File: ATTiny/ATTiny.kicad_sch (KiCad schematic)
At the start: 6 parts

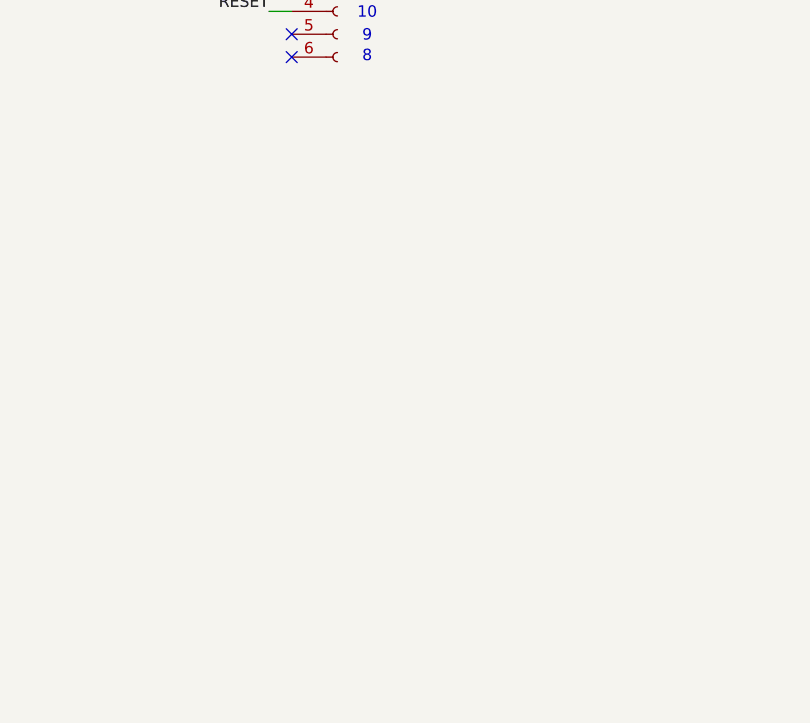
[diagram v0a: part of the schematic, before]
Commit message: header pins complete
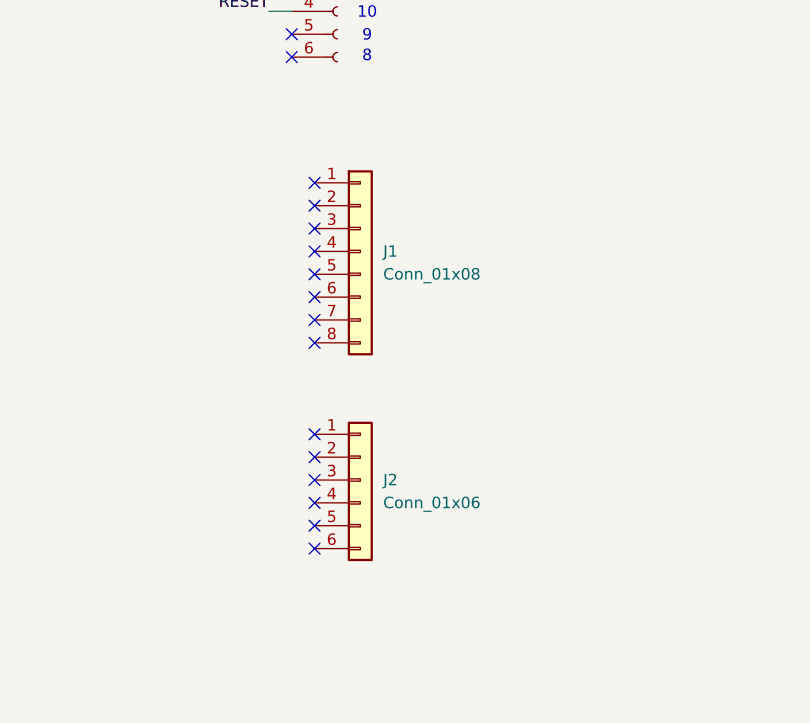
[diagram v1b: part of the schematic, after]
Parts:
- added J1: Conn_01x08, symbol Connector_Generic:Conn_01x08
- added J2: Conn_01x06, symbol Connector_Generic:Conn_01x06
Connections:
- no-connect marks 6 -> 20
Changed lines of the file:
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@@
+	)
+	(no_connect
+		(at 102.87 77.47)
+	)
+	(no_connect
+		(at 102.87 74.93)
+	)
+	(no_connect
+		(at 102.87 92.71)
+	)
+	(no_connect
+		(at 102.87 87.63)
+	)
+	(no_connect
+		(at 102.87 67.31)
+	)
+	(no_connect
+		(at 102.87 95.25)
 	)
 	(no_connect
@@
 	)
 	(no_connect
+		(at 102.87 69.85)
+	)
+	(no_connect
+		(at 102.87 59.69)
+	)
+	(no_connect
+		(at 102.87 97.79)
+	)
+	(no_connect
+		(at 102.87 72.39)
+	)
+	(no_connect
 		(at 33.02 45.72)
 	)
 	(no_connect
+		(at 102.87 64.77)
+	)
+	(no_connect
 		(at 34.29 90.17)
 	)
 	(no_connect
 		(at 34.29 92.71)
+	)
+	(no_connect
+		(at 102.87 62.23)
+	)
+	(no_connect
+		(at 102.87 90.17)
+	)
+	(no_connect
+		(at 102.87 100.33)
 	)
 	(wire
@@
 					(unit 1)
 				)
+			)
+		)
+	)
+	(symbol
+		(lib_id "Connector_Generic:Conn_01x06")
+		(at 107.95 92.71 0)
+		(unit 1)
+		(body_style 1)
+		(exclude_from_sim no)
+		(in_bom yes)
+		(on_board yes)
+		(in_pos_files yes)
+		(dnp no)
+		(fields_autoplaced yes)
+		(property "Reference" "J2"
+			(at 110.49 92.7099 0)
+			(show_name no)
+			(do_not_autoplace no)
+			(effects
+				(font
+					(size 1.27 1.27)
+				)
+				(justify left)
+			)
+		)
+		(property "Value" "Conn_01x06"
+			(at 110.49 95.2499 0)
+			(show_name no)
+			(do_not_autoplace no)
+			(effects
+				(font
+					(size 1.27 1.27)
+				)
+				(justify left)
+			)
+		)
+		(property "Footprint" ""
+			(at 107.95 92.71 0)
+			(hide yes)
+			(show_name no)
+			(do_not_autoplace no)
+			(effects
+				(font
+					(size 1.27 1.27)
+				)
+			)
+		)
+		(property "Datasheet" ""
+			(at 107.95 92.71 0)
+			(hide yes)
+			(show_name no)
+			(do_not_autoplace no)
+			(effects
+				(font
+					(size 1.27 1.27)
+				)
+			)
+		)
+		(property "Description" "Generic connector, single row, 01x06, script generated (kicad-library-utils/schlib/autogen/connector/)"
+			(at 107.95 92.71 0)
+			(hide yes)
+			(show_name no)
+			(do_not_autoplace no)
+			(effects
+				(font
+					(size 1.27 1.27)
+				)
+			)
+		)
+		(pin "3"
+		)
+		(pin "2"
+		)
+		(pin "1"
+		)
+		(pin "4"
+		)
+		(pin "6"
+		)
+		(pin "5"
+		)
+		(instances
+			(project "ATTiny"
+				(path "/46ef1815-a8ed-4d38-a82f-c72395c084aa"
+					(reference "J2")
+					(unit 1)
+				)
+			)
+		)
+	)
+	(symbol
+		(lib_id "Connector_Generic:Conn_01x08")
+		(at 107.95 67.31 0)
+		(unit 1)
+		(body_style 1)
+		(exclude_from_sim no)
+		(in_bom yes)
+		(on_board yes)
+		(in_pos_files yes)
+		(dnp no)
+		(fields_autoplaced yes)
+		(property "Reference" "J1"
+			(at 110.49 67.3099 0)
+			(show_name no)
+			(do_not_autoplace no)
+			(effects
+				(font
+					(size 1.27 1.27)
+				)
+				(justify left)
+			)
+		)
+		(property "Value" "Conn_01x08"
+			(at 110.49 69.8499 0)
+			(show_name no)
+			(do_not_autoplace no)
+			(effects
+				(font
+					(size 1.27 1.27)
+				)
+				(justify left)
+			)
+		)
+		(property "Footprint" ""
+			(at 107.95 67.31 0)
+			(hide yes)
+			(show_name no)
+			(do_not_autoplace no)
+			(effects
+				(font
+					(size 1.27 1.27)
+				)
+			)
+		)
+		(property "Datasheet" ""
+			(at 107.95 67.31 0)
+			(hide yes)
+			(show_name no)
+			(do_not_autoplace no)
+			(effects
+				(font
+					(size 1.27 1.27)
+				)
+			)
+		)
+		(property "Description" "Generic connector, single row, 01x08, script generated (kicad-library-utils/schlib/autogen/connector/)"
+			(at 107.95 67.31 0)
+			(hide yes)
+			(show_name no)
+			(do_not_autoplace no)
+			(effects
+				(font
+					(size 1.27 1.27)
+				)
+			)
+		)
+		(pin "8"
+		)
+		(pin "7"
+		)
+		(pin "5"
+		)
+		(pin "4"
+		)
+		(pin "1"
+		)
+		(pin "3"
+		)
+		(pin "2"
+		)
+		(pin "6"
+		)
+		(instances
+			(project "ATTiny"
+				(path "/46ef1815-a8ed-4d38-a82f-c72395c084aa"
+					(reference "J1")
+					(unit 1)
+				)

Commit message: return
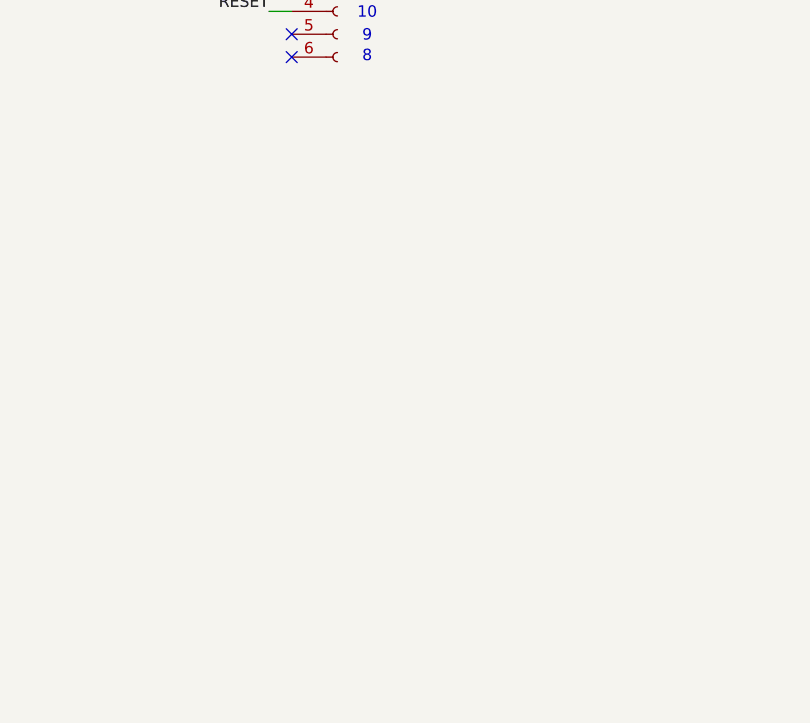
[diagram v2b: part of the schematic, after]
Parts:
- removed J1: Conn_01x08, symbol Connector_Generic:Conn_01x08
- removed J2: Conn_01x06, symbol Connector_Generic:Conn_01x06
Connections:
- no-connect marks 20 -> 6
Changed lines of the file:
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@@
-	)
-	(no_connect
-		(at 102.87 77.47)
-	)
-	(no_connect
-		(at 102.87 74.93)
-	)
-	(no_connect
-		(at 102.87 92.71)
-	)
-	(no_connect
-		(at 102.87 87.63)
-	)
-	(no_connect
-		(at 102.87 67.31)
-	)
-	(no_connect
-		(at 102.87 95.25)
 	)
 	(no_connect
@@
 	)
 	(no_connect
-		(at 102.87 69.85)
-	)
-	(no_connect
-		(at 102.87 59.69)
-	)
-	(no_connect
-		(at 102.87 97.79)
-	)
-	(no_connect
-		(at 102.87 72.39)
-	)
-	(no_connect
 		(at 33.02 45.72)
-	)
-	(no_connect
-		(at 102.87 64.77)
 	)
 	(no_connect
@@
 	(no_connect
 		(at 34.29 92.71)
-	)
-	(no_connect
-		(at 102.87 62.23)
-	)
-	(no_connect
-		(at 102.87 90.17)
-	)
-	(no_connect
-		(at 102.87 100.33)
 	)
 	(wire
@@
 					(unit 1)
 				)
-			)
-		)
-	)
-	(symbol
-		(lib_id "Connector_Generic:Conn_01x06")
-		(at 107.95 92.71 0)
-		(unit 1)
-		(body_style 1)
-		(exclude_from_sim no)
-		(in_bom yes)
-		(on_board yes)
-		(in_pos_files yes)
-		(dnp no)
-		(fields_autoplaced yes)
-		(property "Reference" "J2"
-			(at 110.49 92.7099 0)
-			(show_name no)
-			(do_not_autoplace no)
-			(effects
-				(font
-					(size 1.27 1.27)
-				)
-				(justify left)
-			)
-		)
-		(property "Value" "Conn_01x06"
-			(at 110.49 95.2499 0)
-			(show_name no)
-			(do_not_autoplace no)
-			(effects
-				(font
-					(size 1.27 1.27)
-				)
-				(justify left)
-			)
-		)
-		(property "Footprint" ""
-			(at 107.95 92.71 0)
-			(hide yes)
-			(show_name no)
-			(do_not_autoplace no)
-			(effects
-				(font
-					(size 1.27 1.27)
-				)
-			)
-		)
-		(property "Datasheet" ""
-			(at 107.95 92.71 0)
-			(hide yes)
-			(show_name no)
-			(do_not_autoplace no)
-			(effects
-				(font
-					(size 1.27 1.27)
-				)
-			)
-		)
-		(property "Description" "Generic connector, single row, 01x06, script generated (kicad-library-utils/schlib/autogen/connector/)"
-			(at 107.95 92.71 0)
-			(hide yes)
-			(show_name no)
-			(do_not_autoplace no)
-			(effects
-				(font
-					(size 1.27 1.27)
-				)
-			)
-		)
-		(pin "3"
-		)
-		(pin "2"
-		)
-		(pin "1"
-		)
-		(pin "4"
-		)
-		(pin "6"
-		)
-		(pin "5"
-		)
-		(instances
-			(project "ATTiny"
-				(path "/46ef1815-a8ed-4d38-a82f-c72395c084aa"
-					(reference "J2")
-					(unit 1)
-				)
-			)
-		)
-	)
-	(symbol
-		(lib_id "Connector_Generic:Conn_01x08")
-		(at 107.95 67.31 0)
-		(unit 1)
-		(body_style 1)
-		(exclude_from_sim no)
-		(in_bom yes)
-		(on_board yes)
-		(in_pos_files yes)
-		(dnp no)
-		(fields_autoplaced yes)
-		(property "Reference" "J1"
-			(at 110.49 67.3099 0)
-			(show_name no)
-			(do_not_autoplace no)
-			(effects
-				(font
-					(size 1.27 1.27)
-				)
-				(justify left)
-			)
-		)
-		(property "Value" "Conn_01x08"
-			(at 110.49 69.8499 0)
-			(show_name no)
-			(do_not_autoplace no)
-			(effects
-				(font
-					(size 1.27 1.27)
-				)
-				(justify left)
-			)
-		)
-		(property "Footprint" ""
-			(at 107.95 67.31 0)
-			(hide yes)
-			(show_name no)
-			(do_not_autoplace no)
-			(effects
-				(font
-					(size 1.27 1.27)
-				)
-			)
-		)
-		(property "Datasheet" ""
-			(at 107.95 67.31 0)
-			(hide yes)
-			(show_name no)
-			(do_not_autoplace no)
-			(effects
-				(font
-					(size 1.27 1.27)
-				)
-			)
-		)
-		(property "Description" "Generic connector, single row, 01x08, script generated (kicad-library-utils/schlib/autogen/connector/)"
-			(at 107.95 67.31 0)
-			(hide yes)
-			(show_name no)
-			(do_not_autoplace no)
-			(effects
-				(font
-					(size 1.27 1.27)
-				)
-			)
-		)
-		(pin "8"
-		)
-		(pin "7"
-		)
-		(pin "5"
-		)
-		(pin "4"
-		)
-		(pin "1"
-		)
-		(pin "3"
-		)
-		(pin "2"
-		)
-		(pin "6"
-		)
-		(instances
-			(project "ATTiny"
-				(path "/46ef1815-a8ed-4d38-a82f-c72395c084aa"
-					(reference "J1")
-					(unit 1)
-				)
